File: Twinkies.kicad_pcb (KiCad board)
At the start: 2 copper layers, 76.2 x 81.3 mm, 56 parts, among them J1 USB_C_Receptacle_USB2.0, J2 Radio u.fl, J3 GPS u.fl, J4 DM3AT-SF-PEJM5, J5 I2C, J6 Arducam, J7 UART+SPI, J8 SDIO, Q1 UMT3904T106, SW1 RESET, SW2 RESET, SW3 RESET, U1 NCP167BMX330TBG, U10 LTC2990, U2 RP2040_Stamp, U3 RFM95W, U4 MAX-M8Q, U5 DS1339BU+T, U6 ISM330DHCXTR, U7 VEML7700-TT, U8 TLV493D, U9 BME280, Y1 32.768kHz

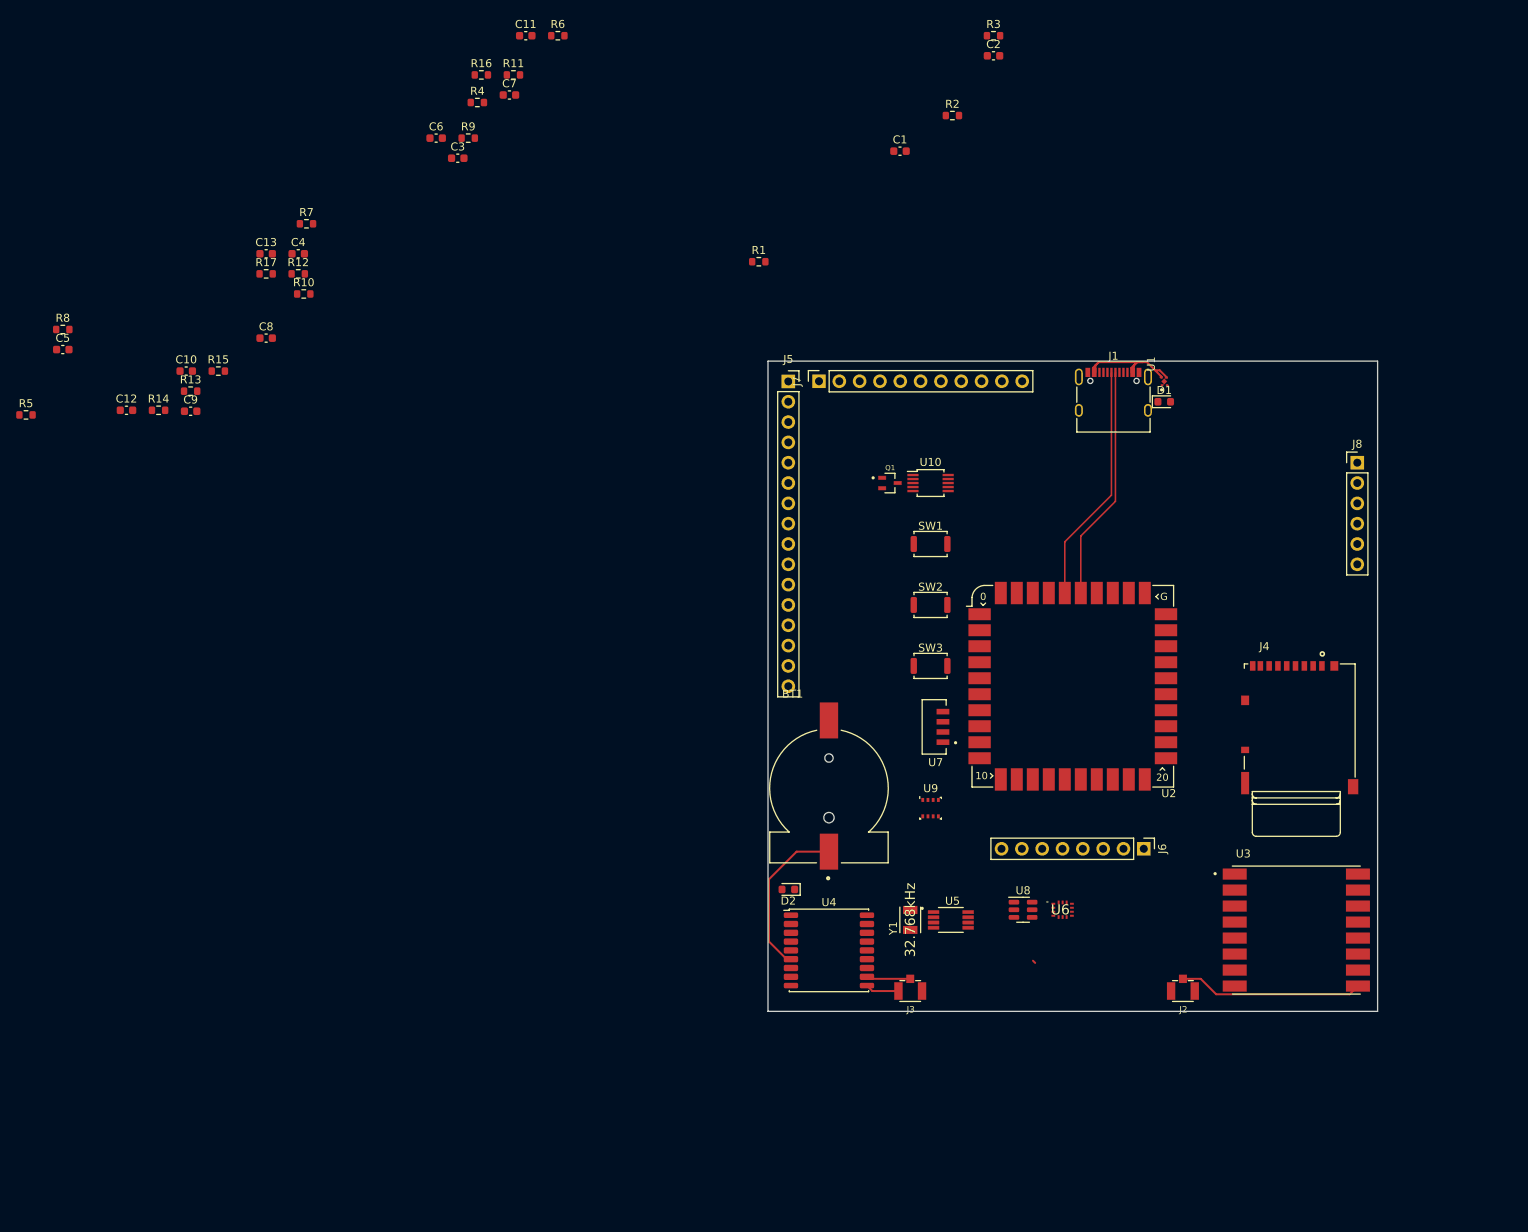
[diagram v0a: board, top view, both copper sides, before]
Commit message: pdu design
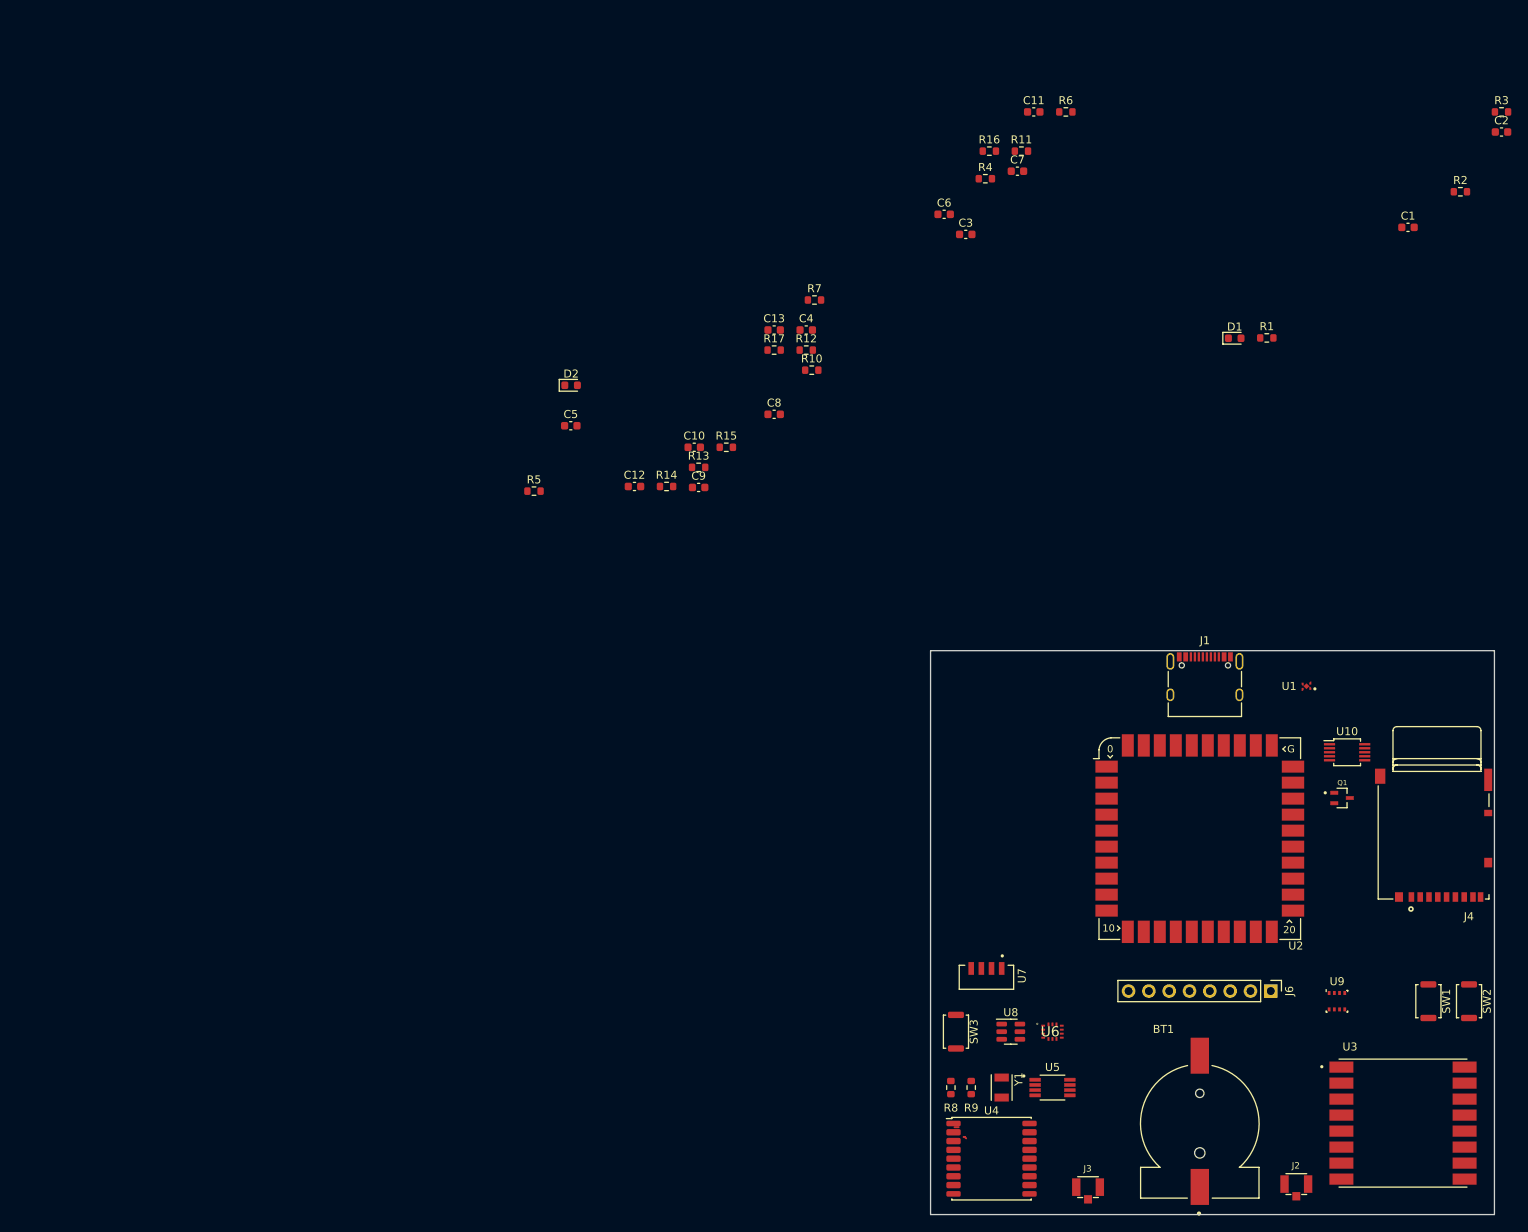
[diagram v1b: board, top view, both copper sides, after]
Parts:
- removed J5: I2C, Connector_PinSocket_2.54mm:PinSocket_1x16_P2.54mm_Vertical
- removed J7: UART+SPI, Connector_PinSocket_2.54mm:PinSocket_1x11_P2.54mm_Vertical
- removed J8: SDIO, Connector_PinHeader_2.54mm:PinHeader_1x06_P2.54mm_Vertical
- SW2: value RESET -> BOOTSEL
- moved R8 146.0 mm to (132.1, 146.7), turned to -90 degrees
- moved R9 134.3 mm to (134.6, 146.7), turned to -90 degrees
- moved SW1 84.5 mm to (191.8, 135.9), turned to -90 degrees
- moved SW2 83.6 mm to (196.8, 135.9), turned to -90 degrees
- moved Q1 68.9 mm to (181.0, 110.5)
- moved D2 68.6 mm to (84.6, 58.9), turned to 0 degrees
- moved C6 64.2 mm to (131.2, 37.5)
- moved C1 64.2 mm to (189.2, 39.2)
- moved C10 64.2 mm to (100.0, 66.7)
- moved C11 64.2 mm to (142.4, 24.7)
- moved C12 64.2 mm to (92.5, 71.5)
- moved C2 64.2 mm to (200.9, 27.2)
- moved C3 64.2 mm to (133.9, 40.0)
- moved C4 64.2 mm to (114.0, 52.0)
- moved C7 64.2 mm to (140.4, 32.1)
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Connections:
- J6 pad 5: RFM_SCK -> CAM_SCK
- J6 pad 6: RFM_MISO -> CAM_MISO
- J6 pad 7: RFM_MOSI -> CAM_MOSI
- U2 pad 10: CAM_SCL -> RTC_SCL
- U2 pad 11: MAG_SDA -> GNSS_SDA
- U2 pad 12: MAG_SCL -> CAM_MOSI
- U2 pad 13: RTC_SDA -> CAM_MISO
- U2 pad 14: RTC_SCL -> CAM_CS
- U2 pad 15: GNSS_SDA -> CAM_SCK
- U2 pad 16: GNSS_SCL -> CAM_SCL
- U2 pad 17: BME_SDA -> CAM_SDA
- U2 pad 18: BME_SCL -> RFM_CS
- U2 pad 19: RFM_SCK -> RFM_RESET
- U2 pad 20: RFM_MOSI -> SDIO_DAT1
- U2 pad 21: RFM_MISO -> SDIO_DAT0
- U2 pad 22: RFM_CS -> SDIO_CLK
- U2 pad 23: CAM_CS -> SDIO_CMD
- U2 pad 24: RFM_RESET -> SDIO_DAT3
- U2 pad 25: SDIO_CMD -> SDIO_DAT2
- U2 pad 26: SDIO_CLK -> GNSS_SCL
- U2 pad 27: SDIO_DAT0 -> BME_SDA
- U2 pad 28: SDIO_DAT1 -> BME_SCL
- U2 pad 29: SDIO_DAT2 -> PWR_SDA
- U2 pad 30: SDIO_DAT3 -> PWR_SCL
- U2 pad 5: PWR_SDA -> LTR_SDA
- U2 pad 6: PWR_SCL -> LTR_SCL
- U2 pad 7: LTR_SDA -> MAG_SDA
- U2 pad 8: LTR_SCL -> MAG_SCL
- U2 pad 9: CAM_SDA -> RTC_SDA
- U3 pad 2: RFM_MISO -> CAM_MISO
- U3 pad 3: RFM_MOSI -> CAM_MOSI
- U3 pad 4: RFM_SCK -> CAM_SCK
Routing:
- net USB_D+: track 30.0 -> 0.00 mm
- net USB_D-: track 29.4 -> 0.00 mm
- net Net-(J2-Pad2): track 23.1 -> 0.00 mm
- net +BATT: track 20.4 -> 0.00 mm
- net VBUS: track 17.4 -> 0.00 mm
- net Net-(J3-Pad2): track 5.52 -> 0.00 mm
- net GND: track 4.22 -> 0.51 mm
- net unconnected-(U2-Pad32): track 0.00 -> 0.65 mm
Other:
- board size 76.2 x 81.3 mm -> 70.5 x 70.5 mm

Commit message: Apr 8
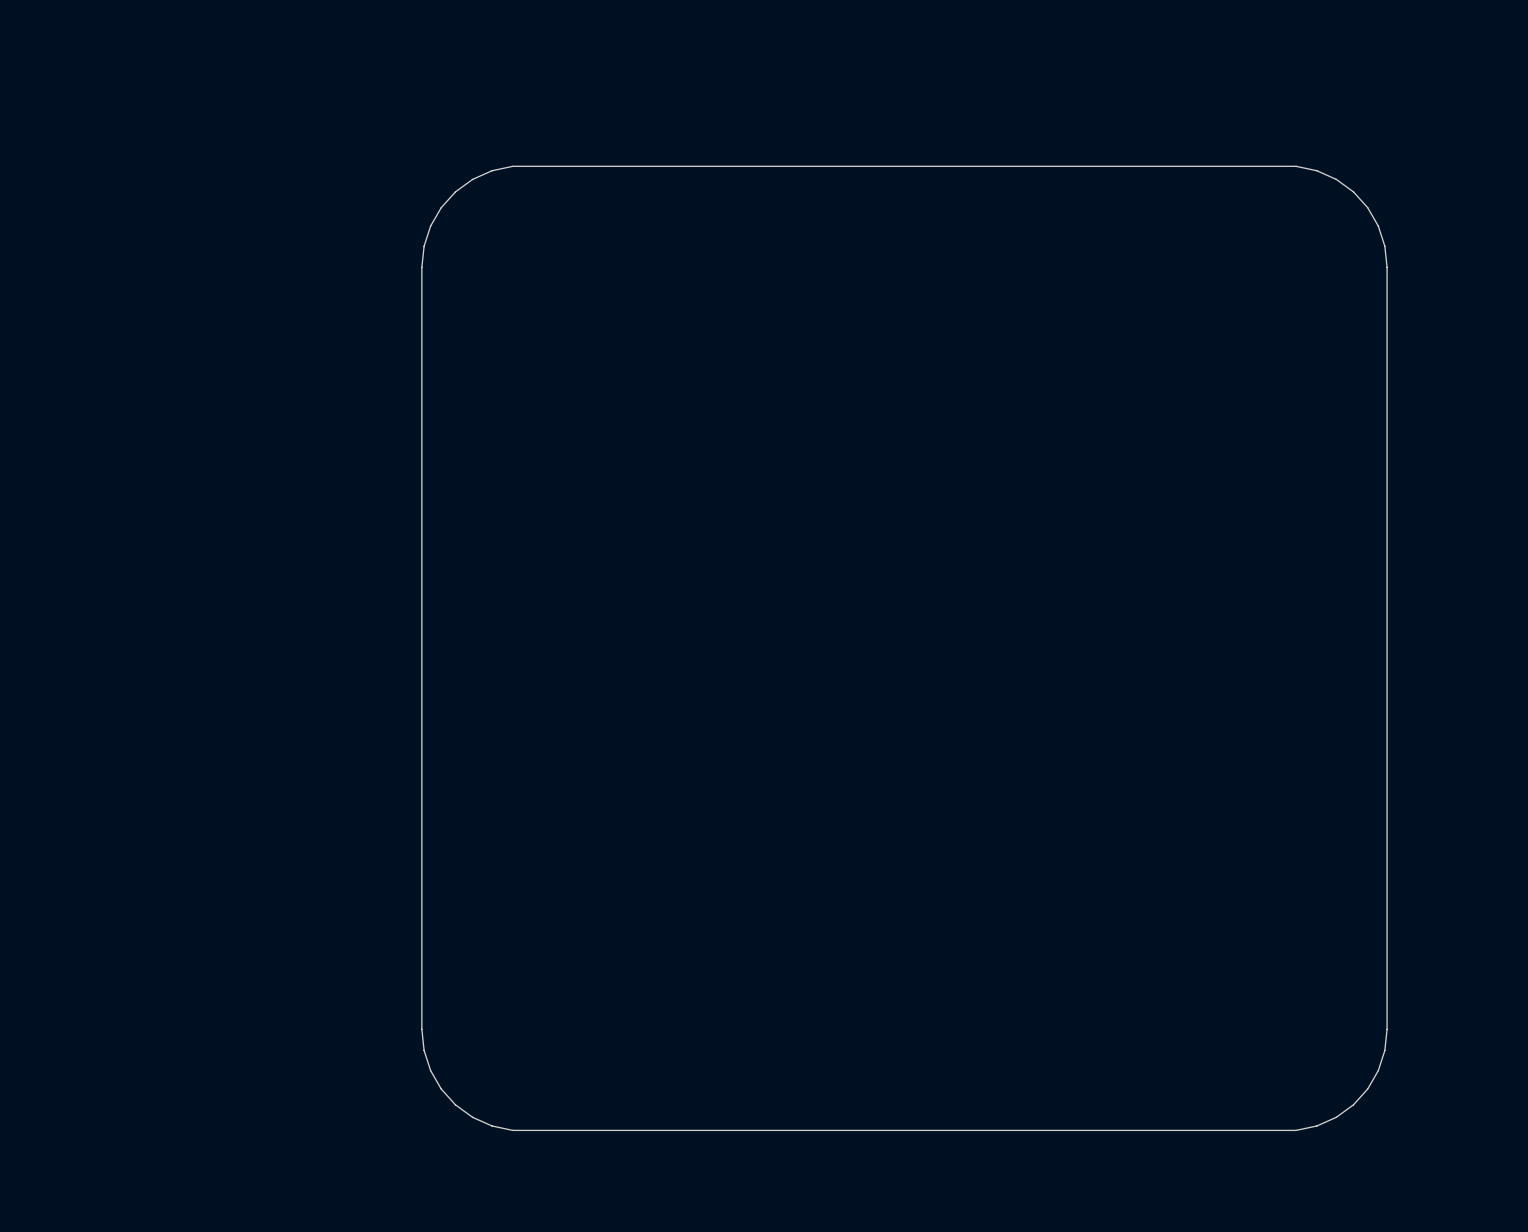
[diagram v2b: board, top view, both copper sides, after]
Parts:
- removed BT1: S8411-45R, S8411-45R:BAT_S8411-45R
- removed C1, C10, C11, C12, C2, C3, C4, C5, C6, C7, C9: 1uF, Capacitor_SMD:C_0603_1608Metric
- removed C13: 470pF, Capacitor_SMD:C_0603_1608Metric
- removed C8: 100nF, Capacitor_SMD:C_0603_1608Metric
- removed D1: PWR, LED_SMD:LED_0603_1608Metric
- removed D2: LED, LED_SMD:LED_0603_1608Metric
- removed J1: USB_C_Receptacle_USB2.0, Connector_USB:USB_C_Receptacle_XKB_U262-16XN-4BVC11
- removed J2: Radio u.fl, u.fl:HRS_U.FL-R-SMT-1(10)
- removed J3: GPS u.fl, u.fl:HRS_U.FL-R-SMT-1(10)
- removed J4: DM3AT-SF-PEJM5, DM3AT-SF-PEJM5:HRS_DM3AT-SF-PEJM5
- removed J6: Arducam, Connector_PinHeader_2.54mm:PinHeader_1x08_P2.54mm_Vertical
- removed Q1: UMT3904T106, SOT65:SOT65P210X100-3N
- removed R1, R10: 1k, Resistor_SMD:R_0603_1608Metric
- removed R11, R12, R13, R14, R4, R5, R6, R7: 10k, Resistor_SMD:R_0603_1608Metric
- removed R15, R16: 4.7k, Resistor_SMD:R_0603_1608Metric
- removed R17: 1, Resistor_SMD:R_0603_1608Metric
- removed R2, R3: 5.1K, Resistor_SMD:R_0603_1608Metric
- removed R8, R9: 470, Resistor_SMD:R_0603_1608Metric
- removed SW1, SW3: RESET, Button_Switch_SMD:SW_Push_SPST_NO_Alps_SKRK
- removed SW2: BOOTSEL, Button_Switch_SMD:SW_Push_SPST_NO_Alps_SKRK
- removed U1: NCP167BMX330TBG, NCP167BMX330TBG:REG_NCP167BMX330TBG
- removed U10: LTC2990, Package_SO:MSOP-10_3x3mm_P0.5mm
- removed U2: RP2040_Stamp, RP2040_Stamp:RP2040_Stamp_SMD
- removed U3: RFM95W, RFM95W-915S2:XCVR_RFM95W-915S2
- removed U4: MAX-M8Q, RF_GPS:ublox_MAX
- removed U5: DS1339BU+T, DS1339BU_T:SOP65P490X110-8N
- removed U6: ISM330DHCXTR, ISM330DHCXTR:LGA-14_2.5X3X0.86_
- removed U7: VEML7700-TT, VEML7700-TT:XDCR_VEML7700-TT
- removed U8: TLV493D, Package_TO_SOT_SMD:SOT-23-6
- removed U9: BME280, Package_LGA:Bosch_LGA-8_2.5x2.5mm_P0.65mm_ClockwisePinNumbering
- removed Y1: 32.768kHz, eec:Abracon-ABS07-120-0-0-MFG
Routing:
- net unconnected-(U2-Pad32): track 0.65 -> 0.00 mm
- net GND: track 0.51 -> 0.00 mm
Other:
- board size 70.5 x 70.5 mm -> 120.6 x 120.5 mm
